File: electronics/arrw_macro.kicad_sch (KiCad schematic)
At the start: 23 parts, among them J7 Conn_01x05_Female, J8 Conn_01x05_Male, SW59 SW_SPST, SW60 SW_SPST, SW61 SW_SPST, SW62 SW_SPST, SW63 SW_SPST, SW64 SW_SPST, SW65 SW_SPST, SW66 SW_SPST, SW67 SW_SPST, SW68 SW_SPST, U4 PCA9675PW

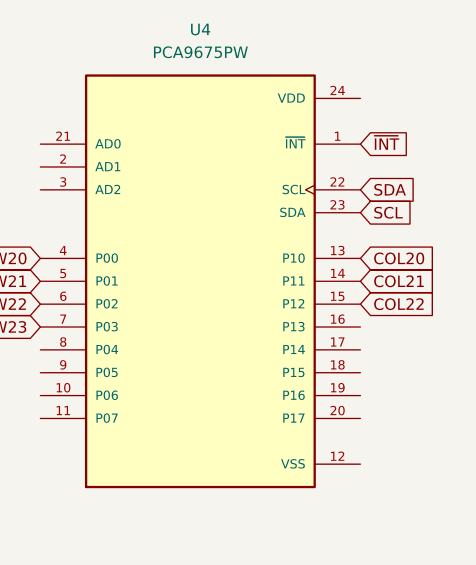
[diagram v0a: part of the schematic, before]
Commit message: finish matrix
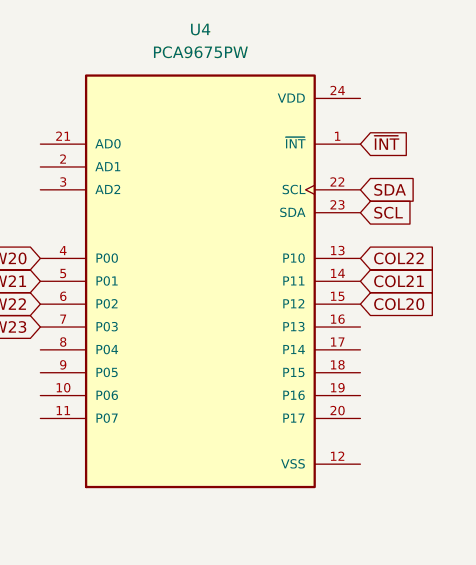
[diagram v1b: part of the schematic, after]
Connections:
- net COL20: now also U4.15 (P12); no longer U4.13 (P10)
- net COL22: now also U4.13 (P10); no longer U4.15 (P12)
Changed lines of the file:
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@@
     (stroke (width 0) (type default) (color 0 0 0 0))
-  )
-  (global_label "COL22" (shape input) (at 224.79 59.69 0) (fields_autoplaced)
-    (effects (font (size 1.27 1.27)) (justify left))
-    (property "Intersheet References" "${INTERSHEET_REFS}" (id 0) (at 233.2507 59.7694 0)
-      (effects (font (size 1.27 1.27)) (justify left) hide)
-    )
   )
   (global_label "ROW22" (shape input) (at 189.23 59.69 180) (fields_autoplaced)
@@
     (property "Intersheet References" "${INTERSHEET_REFS}" (id 0) (at 54.6159 121.8406 0)
       (effects (font (size 1.27 1.27)) (justify right) hide)
+    )
+  )
+  (global_label "COL21" (shape input) (at 224.79 57.15 0) (fields_autoplaced)
+    (effects (font (size 1.27 1.27)) (justify left))
+    (property "Intersheet References" "${INTERSHEET_REFS}" (id 0) (at 233.2507 57.0706 0)
+      (effects (font (size 1.27 1.27)) (justify left) hide)
     )
   )
@@
     )
   )
+  (global_label "COL20" (shape input) (at 224.79 59.69 0) (fields_autoplaced)
+    (effects (font (size 1.27 1.27)) (justify left))
+    (property "Intersheet References" "${INTERSHEET_REFS}" (id 0) (at 233.2507 59.6106 0)
+      (effects (font (size 1.27 1.27)) (justify left) hide)
+    )
+  )
   (global_label "ROW21" (shape input) (at 104.14 121.92 180) (fields_autoplaced)
     (effects (font (size 1.27 1.27)) (justify right))
@@
     (property "Intersheet References" "${INTERSHEET_REFS}" (id 0) (at 54.6159 106.6006 0)
       (effects (font (size 1.27 1.27)) (justify right) hide)
-    )
-  )
-  (global_label "COL20" (shape input) (at 224.79 54.61 0) (fields_autoplaced)
-    (effects (font (size 1.27 1.27)) (justify left))
-    (property "Intersheet References" "${INTERSHEET_REFS}" (id 0) (at 233.2507 54.6894 0)
-      (effects (font (size 1.27 1.27)) (justify left) hide)
     )
   )
@@
     )
   )
-  (global_label "COL21" (shape input) (at 224.79 57.15 0) (fields_autoplaced)
-    (effects (font (size 1.27 1.27)) (justify left))
-    (property "Intersheet References" "${INTERSHEET_REFS}" (id 0) (at 233.2507 57.2294 0)
-      (effects (font (size 1.27 1.27)) (justify left) hide)
-    )
-  )
   (global_label "ROW23" (shape input) (at 104.14 170.18 180) (fields_autoplaced)
     (effects (font (size 1.27 1.27)) (justify right))
@@
       (effects (font (size 1.27 1.27)) (justify left) hide)
     )
+  )
+  (global_label "COL22" (shape input) (at 224.79 54.61 0) (fields_autoplaced)
+    (effects (font (size 1.27 1.27)) (justify left))
+    (property "Intersheet References" "${INTERSHEET_REFS}" (id 0) (at 233.2507 54.5306 0)
+      (effects (font (size 1.27 1.27)) (justify left) hide)
+    )
